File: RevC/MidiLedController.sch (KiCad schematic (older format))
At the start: 53 parts, among them J1 Molex 2Way KK254, J12 Barrel_Jack, SW1 SW_DIP_x04, SW2 SW_SPST, U20 STM32F051K8Tx, U21 6N135S

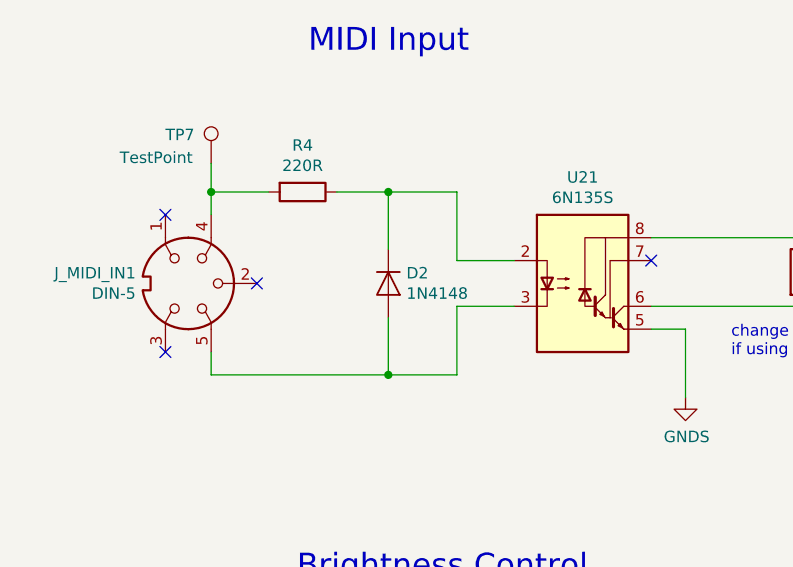
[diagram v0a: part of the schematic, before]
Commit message: updates
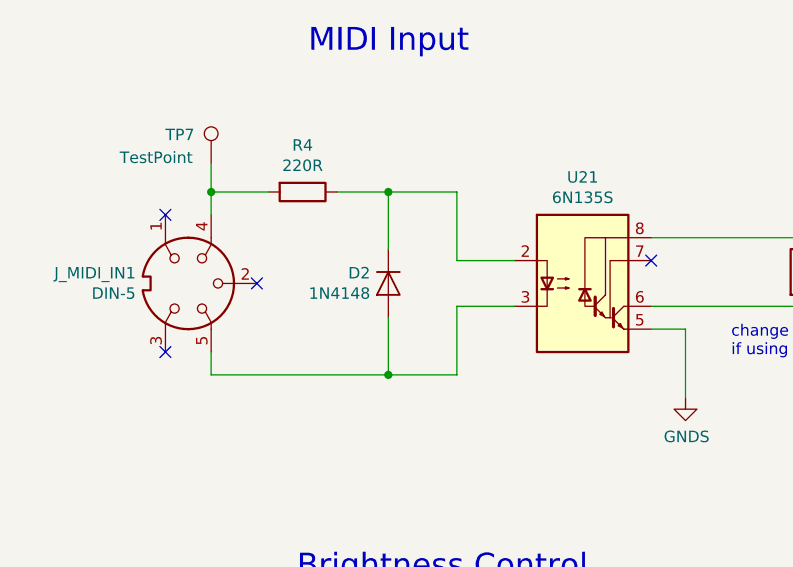
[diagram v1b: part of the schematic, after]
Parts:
- C26, C5: LcscNo (none) -> C152892; MouserNo 710-885012207027 -> (none); Type (none) -> N/A
- C28, C6: LcscNo (none) -> C94108; MouserNo 710-885012207098 -> (none); Type (none) -> N/A
- C32: LcscNo (none) -> C87998; MouserNo 791-0805X475M250CT -> (none); Type (none) -> N/A
- C33: LcscNo (none) -> C107135; MouserNo 710-885012207066 -> (none); Type (none) -> N/A
- C34: LcscNo (none) -> C376927; MouserNo 791-0805X105K100CT -> (none); Type (none) -> N/A
- D2, R4, R9: Type (none) -> N/A
- D_STATUS1, D_STATUS_2, D_STATUS_3, D_STATUS_4, D_STATUS_5, D_STATUS_6, D_STATUS_7, D_STATUS_8, D_STATUS_9, J1, J_AUX1, J_OUT1, J_OUT2, J_OUT3, J_OUT4, J_OUT5, J_OUT6, J_OUT7, J_OUT8, J_OUT9, SW1, SW2: EbayPurchase (none) -> True
- J12: EbayPurchase (none) -> True; MouserNo 502-RAPC722X -> (none)
- J_MIDI_IN1: EbayPurchase (none) -> True; RSComponentsNo 491-087 -> (none)
- R1: LcscNo (none) -> C115295; MouserNo 71-CRCW080510K0FKEAC -> (none); Type (none) -> N/A
- R119, R120, R121, R122: LcscNo (none) -> C25623; Type (none) -> N/A
- R25, R74: LcscNo (none) -> C106949; MouserNo 71-CRCW0805100RFKEAC -> (none); Type (none) -> N/A
- RV1: MouserNo (none) -> 652-PTH901-030S-103B; Type (none) -> PTH901-030S-103B1
- RV1: MouserNo (none) -> 652-PTH901-030S-103B; Type (none) -> PTH901-030S-103B
